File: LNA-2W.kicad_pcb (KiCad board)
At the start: 2 copper layers, 58.2 x 30 mm, 30 parts, among them J1 SMA_Edge, J2 SMA_Edge, U1 TQP7M9106

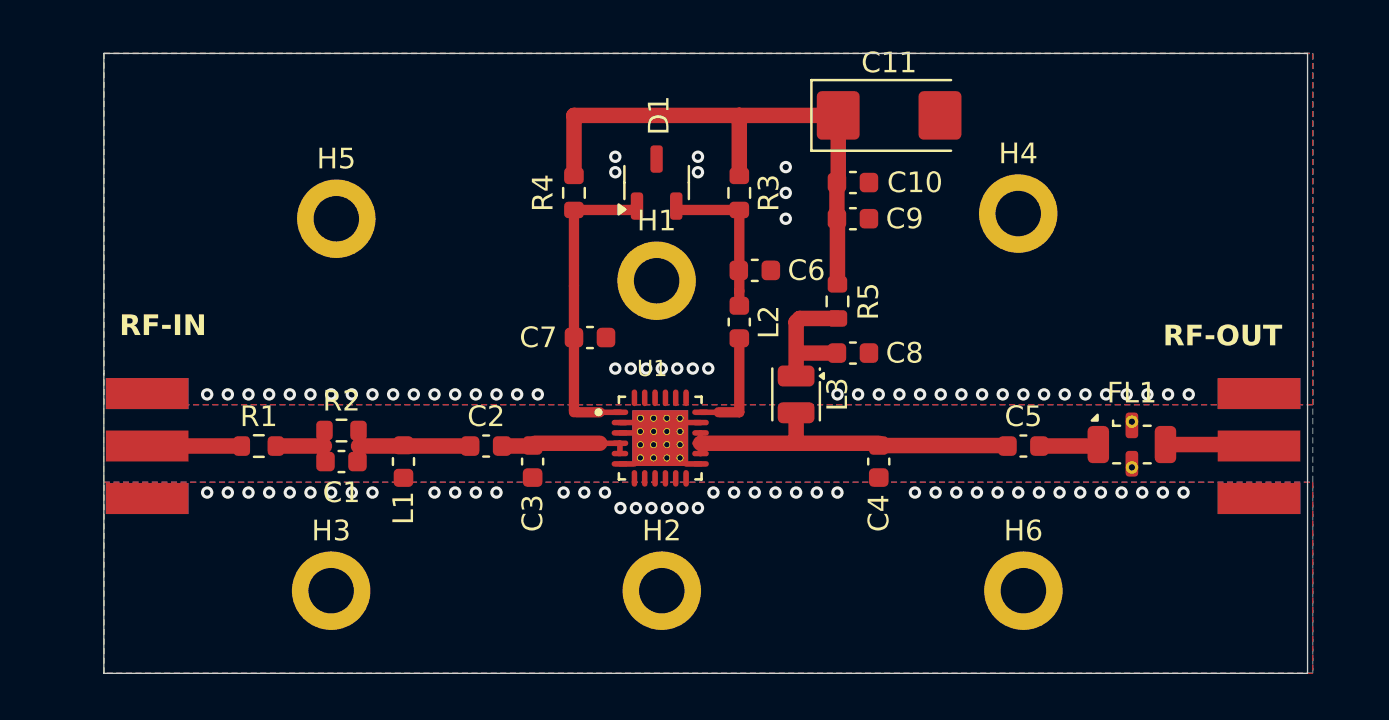
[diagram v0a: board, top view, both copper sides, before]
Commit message: Add files via upload
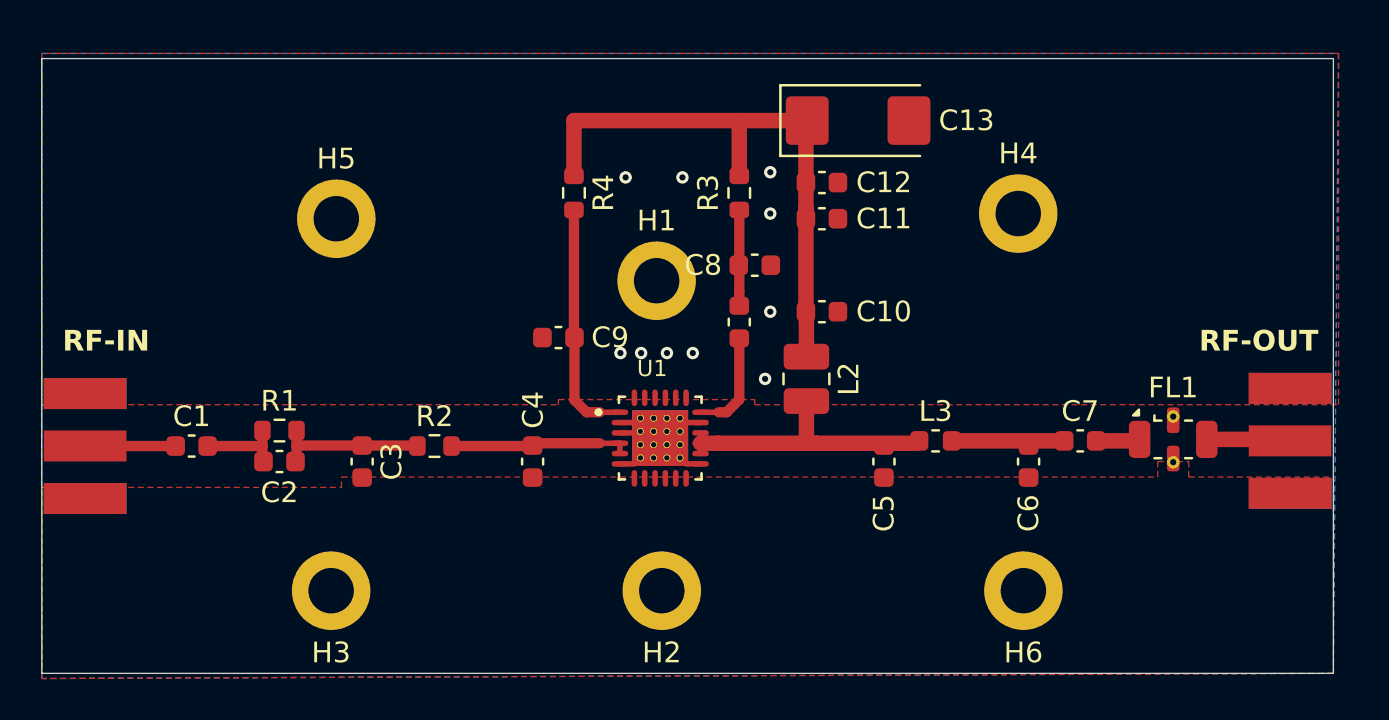
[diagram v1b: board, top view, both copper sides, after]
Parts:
- removed D1: SM05T1G, Package_TO_SOT_SMD:SOT-23-3
- removed R5: 0R, Resistor_SMD:R_0603_1608Metric
- added C12: 1n, Capacitor_SMD:C_0603_1608Metric, F.Cu at (142.8, 96.2)
- added C13: 10u, Capacitor_Tantalum_SMD:CP_EIA-6032-28_Kemet-C, F.Cu at (144.5, 93.2)
- C1: value 22p -> 100p
- C11: value 10u -> 100p; footprint Capacitor_Tantalum_SMD:CP_EIA-6032-28_Kemet-C -> Capacitor_SMD:C_0603_1608Metric
- C2: value 2p4 -> 100p
- C3: value 6p8 -> 8p2
- C4: value 8p2 -> 15p
- C5: value 100p -> 8p2
- C6: value 100n -> 6p8
- C7: value 100p -> 22p
- J1: value SMA_Edge -> SMA_RF IN
- J2: value SMA_Edge -> SMA_RF OUT
- L1: value 8n2 -> 68n
- L2: value 68n -> 18n; footprint Inductor_SMD:L_0603_1608Metric -> Inductor_SMD:L_1008_2520Metric
- L3: value 18n -> 4n7; footprint Inductor_SMD:L_Coilcraft_0805HQ_2012Metric -> Inductor_SMD:L_0603_1608Metric
- R1: value 0R -> 51R
- R2: value 51R -> 4R3
- R3: value 240R -> 280R
- moved C7 24.2 mm to (155.2, 108.8), turned to 0 degrees
- moved L1 17.6 mm to (138.8, 103.0)
- moved C4 16.8 mm to (128.8, 109.8)
- moved C6 16.2 mm to (152.8, 109.8), turned to 90 degrees
- moved C9 15.4 mm to (130.0, 103.8)
- moved C2 10.0 mm to (116.5, 109.8)
- moved C3 8.25 mm to (120.5, 109.8)
- moved C1 7.29 mm to (112.2, 109.0)
- moved L3 7.12 mm to (148.2, 108.8), turned to 0 degrees
- moved C5 6.79 mm to (145.8, 109.8), turned to -90 degrees
- moved C10 6.43 mm to (142.8, 102.5)
- moved C8 6.37 mm to (139.5, 100.2), turned to 180 degrees
- moved C11 5.96 mm to (142.8, 98.0)
- moved R2 4.56 mm to (124.0, 109.0)
- moved L2 4.26 mm to (142.0, 105.8)
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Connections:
- C1 pad 1: Net-(C1-Pad1) -> Net-(J1-In)
- C5 pad 1: Net-(C4-Pad1) -> Net-(C5-Pad1)
- C5 pad 2: Net-(FL1-IN) -> GND
- C7 pad 1: GND -> Net-(C6-Pad2)
- C7 pad 2: Net-(U1-VBIAS) -> Net-(FL1-IN)
- C8 pad 1: Net-(C8-Pad1) -> GND
- C8 pad 2: GND -> Net-(C8-Pad2)
- C9 pad 1: +5V -> GND
- C9 pad 2: GND -> Net-(U1-VBIAS)
- L1 pad 1: Net-(C1-Pad2) -> Net-(C8-Pad2)
- L1 pad 2: GND -> Net-(U1-I_REF)
- L2 pad 1: Net-(C6-Pad2) -> +5V
- L2 pad 2: Net-(U1-I_REF) -> Net-(C5-Pad1)
- L3 pad 1: Net-(C8-Pad1) -> Net-(C5-Pad1)
- L3 pad 2: Net-(C4-Pad1) -> Net-(C6-Pad2)
- R1 pad 1: Net-(J1-In) -> Net-(C1-Pad2)
- R1 pad 2: Net-(C1-Pad1) -> Net-(C2-Pad2)
- R2 pad 1: Net-(C1-Pad1) -> Net-(C2-Pad2)
- R2 pad 2: Net-(C1-Pad2) -> Net-(C4-Pad1)
- R3 pad 2: Net-(C6-Pad2) -> Net-(C8-Pad2)
- U1 pad 14: Net-(C4-Pad1) -> Net-(C5-Pad1)
- U1 pad 15: Net-(C4-Pad1) -> Net-(C5-Pad1)
- U1 pad 16: Net-(C4-Pad1) -> Net-(C5-Pad1)
- U1 pad 4: Net-(C2-Pad2) -> Net-(C4-Pad1)
- U1 pad 5: Net-(C2-Pad2) -> Net-(C4-Pad1)
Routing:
- net Net-(C5-Pad1): track 0.00 -> 13.9 mm
- net Net-(C4-Pad1): track 17.3 -> 8.90 mm
- net Net-(C8-Pad1): track 6.44 -> 0.00 mm
- net Net-(C8-Pad2): track 0.00 -> 4.80 mm
- net Net-(C1-Pad1): track 3.87 -> 0.00 mm
- net Net-(U1-VBIAS): track 15.2 -> 11.8 mm
- net Net-(C1-Pad2): track 6.77 -> 4.17 mm
- net Net-(C6-Pad2): track 7.92 -> 5.44 mm
- net +5V: track 26.8 -> 28.1 mm
- net Net-(C2-Pad2): track 6.41 -> 7.39 mm
- net Net-(FL1-IN): track 2.88 -> 2.23 mm
- net GND: vias 92 -> 10
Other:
- board size 58.2 x 30 mm -> 62.5 x 29.8 mm
